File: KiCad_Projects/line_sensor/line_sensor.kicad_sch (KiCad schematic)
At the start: 4 parts, among them J1 Conn_01x05_Female, U1 S4282-51, U2 S4282-51

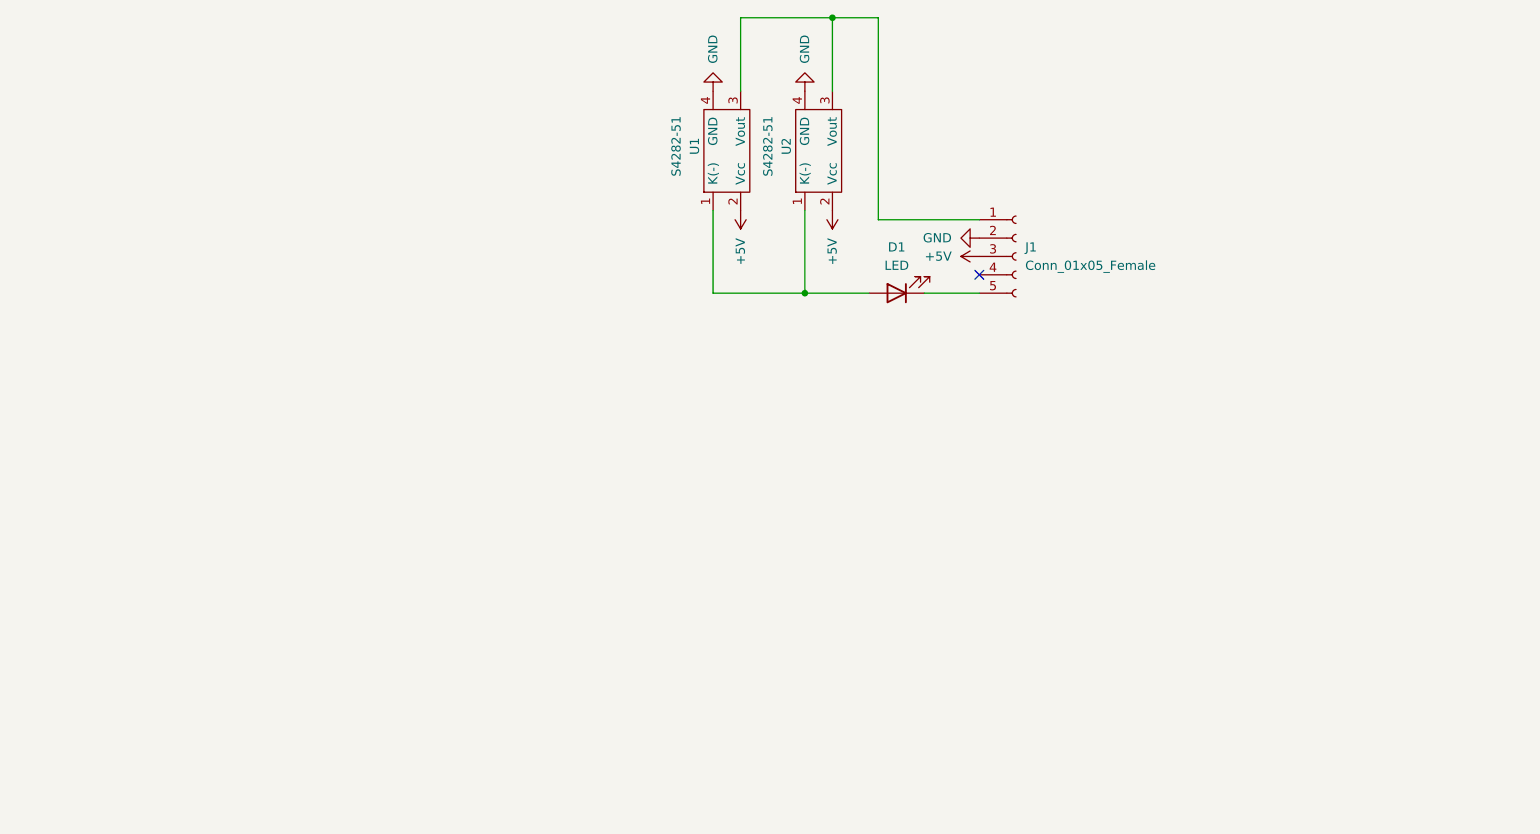
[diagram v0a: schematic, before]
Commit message: 基盤データのアップデート
ローカルコミットはちゃんと作ってください
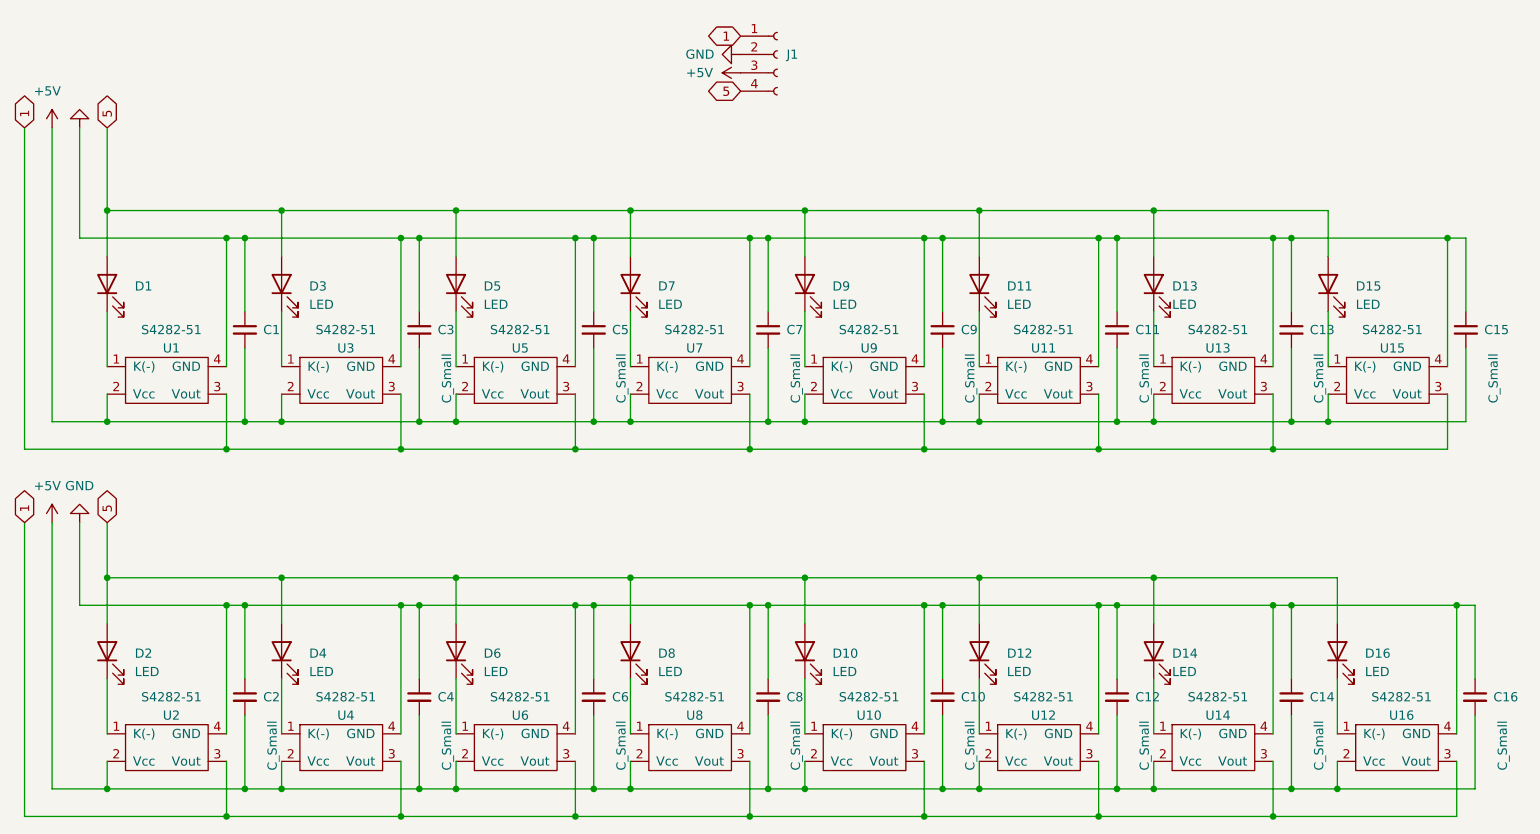
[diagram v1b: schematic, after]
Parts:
- removed J1: Conn_01x05_Female, Connector_PinHeader_2.54mm:PinHeader_1x05_P2.54mm_Vertical, symbol Connector:Conn_01x05_Female
- added C1: (no value), symbol Device:C_Small
- added C10, C11, C12, C13, C14, C15, C16, C2, C3, C4, C5, C6, C7, C8, C9: C_Small, symbol Device:C_Small
- added D10, D11, D12, D13, D14, D15, D16, D2, D3, D4, D5, D6, D7, D8, D9: LED, symbol Device:LED
- added J1: (no value), symbol Connector:Conn_01x04_Female
- added U10, U11, U12, U13, U14, U15, U16, U3, U4, U5, U6, U7, U8, U9: S4282-51, symbol New_Library:S4282-51
- D1: value LED -> (none); footprint LED_THT:LED_D3.0mm_Clear -> (none)
- U1, U2: footprint line_sensor:S4282-51 -> (none)
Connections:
- net +5V: now also C1.2, C10.2, C11.2, C12.2, C13.2, C14.2, C15.2, C16.2, C2.2, C3.2, C4.2, C5.2, C6.2, C7.2, C8.2, C9.2, J1.3 (Pin_3), U10.2 (Vcc), U11.2 (Vcc), U12.2 (Vcc), U13.2 (Vcc), U14.2 (Vcc), U15.2 (Vcc), U16.2 (Vcc), U3.2 (Vcc), U4.2 (Vcc), U5.2 (Vcc), U6.2 (Vcc), U7.2 (Vcc), U8.2 (Vcc), U9.2 (Vcc)
- net GND: now also C1.1, C10.1, C11.1, C12.1, C13.1, C14.1, C15.1, C16.1, C2.1, C3.1, C4.1, C5.1, C6.1, C7.1, C8.1, C9.1, J1.2 (Pin_2), U10.4 (GND), U11.4 (GND), U12.4 (GND), U13.4 (GND), U14.4 (GND), U15.4 (GND), U16.4 (GND), U3.4 (GND), U4.4 (GND), U5.4 (GND), U6.4 (GND), U7.4 (GND), U8.4 (GND), U9.4 (GND)
- net 1: now reaches U1.3 (Vout), U2.3 (Vout)
- net 1: now also J1.1 (Pin_1), U10.3 (Vout), U11.3 (Vout), U12.3 (Vout), U13.3 (Vout), U14.3 (Vout), U15.3 (Vout), U16.3 (Vout), U3.3 (Vout), U4.3 (Vout), U5.3 (Vout), U6.3 (Vout), U7.3 (Vout), U8.3 (Vout), U9.3 (Vout)
- net at D1.1 (K): now also U1.1 (K(-))
- new net: D5.1 (K), U5.1 (K(-))
- new net: D12.1 (K), U12.1 (K(-))
- new net: D15.1 (K), U15.1 (K(-))
- new net: D7.1 (K), U7.1 (K(-))
- new net: D3.1 (K), U3.1 (K(-))
- new net: D11.1 (K), U11.1 (K(-))
- new net: D13.1 (K), U13.1 (K(-))
- new net: D2.1 (K), U2.1 (K(-))
- new net: D8.1 (K), U8.1 (K(-))
- new net: D9.1 (K), U9.1 (K(-))
- new net: D16.1 (K), U16.1 (K(-))
- new net: D6.1 (K), U6.1 (K(-))
- new net: D14.1 (K), U14.1 (K(-))
- new net: D10.1 (K), U10.1 (K(-))
- new net: D4.1 (K), U4.1 (K(-))
- new net 5: D1.2 (A), D10.2 (A), D11.2 (A), D12.2 (A), D13.2 (A), D14.2 (A), D15.2 (A), D16.2 (A), D2.2 (A), D3.2 (A), D4.2 (A), D5.2 (A), D6.2 (A), D7.2 (A), D8.2 (A), D9.2 (A), J1.4 (Pin_4)
- no-connect marks 1 -> 0
